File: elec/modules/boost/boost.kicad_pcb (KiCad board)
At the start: 2 copper layers, 40.6 x 61 mm, 9 parts, among them J1 Conn_01x05, J2 Conn_01x05, U1 LM2587S-ADJ

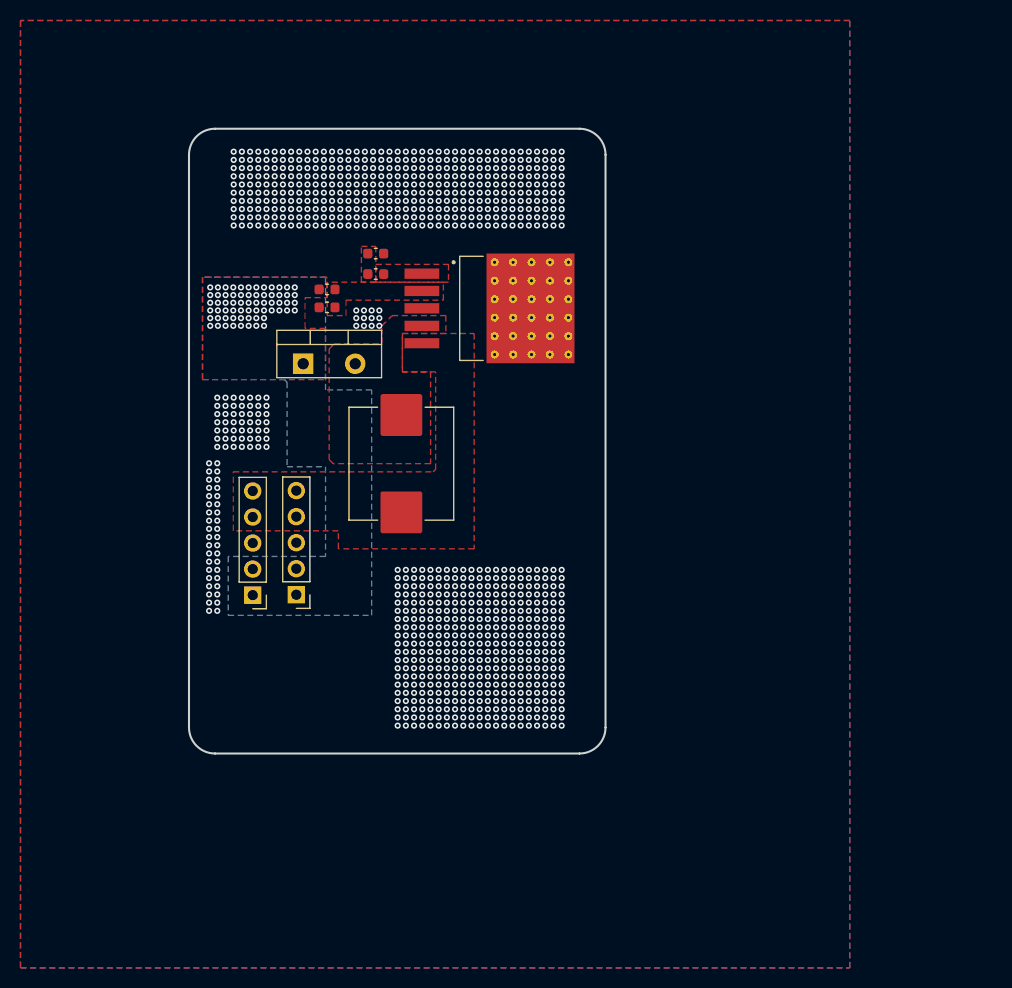
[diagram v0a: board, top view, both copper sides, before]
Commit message: sleepy but did most pcbs
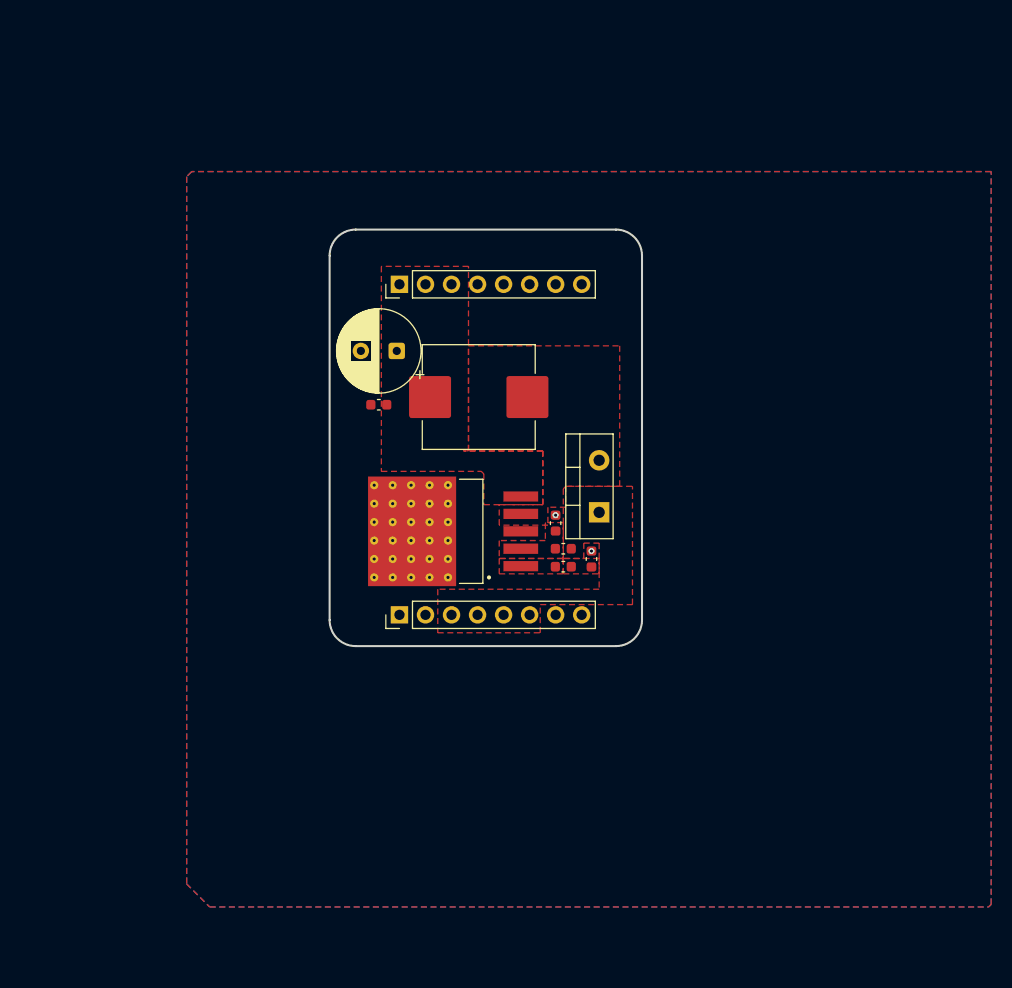
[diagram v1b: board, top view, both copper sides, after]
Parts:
- added C35: 0.1uF, Capacitor_SMD:C_0603_1608Metric, F.Cu at (128.3, 102.9)
- added C36: 100uF, Capacitor_THT:CP_Radial_D8.0mm_P3.50mm, F.Cu at (130.0, 97.6)
- J1, J2: value Conn_01x05 -> Conn_01x08; footprint Pinheaders:PinHeader_1x05_P2.54mm_Vertical -> Pinheaders:PinHeader_1x08_P2.54mm_Vertical
- moved C40 36.5 mm to (149.0, 117.9), turned to 90 degrees
- moved R35 34.2 mm to (146.3, 116.9), turned to 180 degrees
- moved R38 33.9 mm to (146.3, 118.7), turned to 0 degrees
- moved J1 33.5 mm to (130.3, 91.1), turned to 90 degrees
- moved D2 32.3 mm to (149.8, 113.4), turned to 90 degrees
- moved R36 30.7 mm to (145.5, 114.4), turned to 90 degrees
- moved U1 24.6 mm to (131.5, 115.2), turned to 180 degrees
- moved J2 10.3 mm to (130.3, 123.4), turned to 90 degrees
- moved L33 9.96 mm to (138.0, 102.1), turned to 0 degrees
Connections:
- J1 pad 1: +24V -> +12V
- J1 pad 2: +24V -> +12V
- J1 pad 3: GND -> +12V
- J1 pad 4: +12V -> unconnected-(J1-Pin_4-Pad4)
- J1 pad 5: +12V -> unconnected-(J1-Pin_5-Pad5)
- J2 pad 1: +24V -> unconnected-(J2-Pin_1-Pad1)
- J2 pad 2: +24V -> unconnected-(J2-Pin_2-Pad2)
- J2 pad 3: GND -> +24V
- J2 pad 4: +12V -> +24V
- J2 pad 5: +12V -> +24V
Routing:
- net GND: vias 929 -> 2
- net +24V: vias 64 -> 0
- removed copper zone on B.Cu, net +24V
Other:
- board size 40.6 x 61 mm -> 30.5 x 40.6 mm
